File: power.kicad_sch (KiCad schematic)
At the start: 67 parts, among them J1 USB_C_Receptacle_USB2.0_14P, Q2 Q_NMOS_GDS, SW2 SW_SPDT, U12 AT24CS08-STUM, U2 BQ25895RTW, U4 LM1117DT-3.3, U5 MCP4017-xxxxLT, U6 TPS25751DREFR_C30169739, U7 LM3478MA

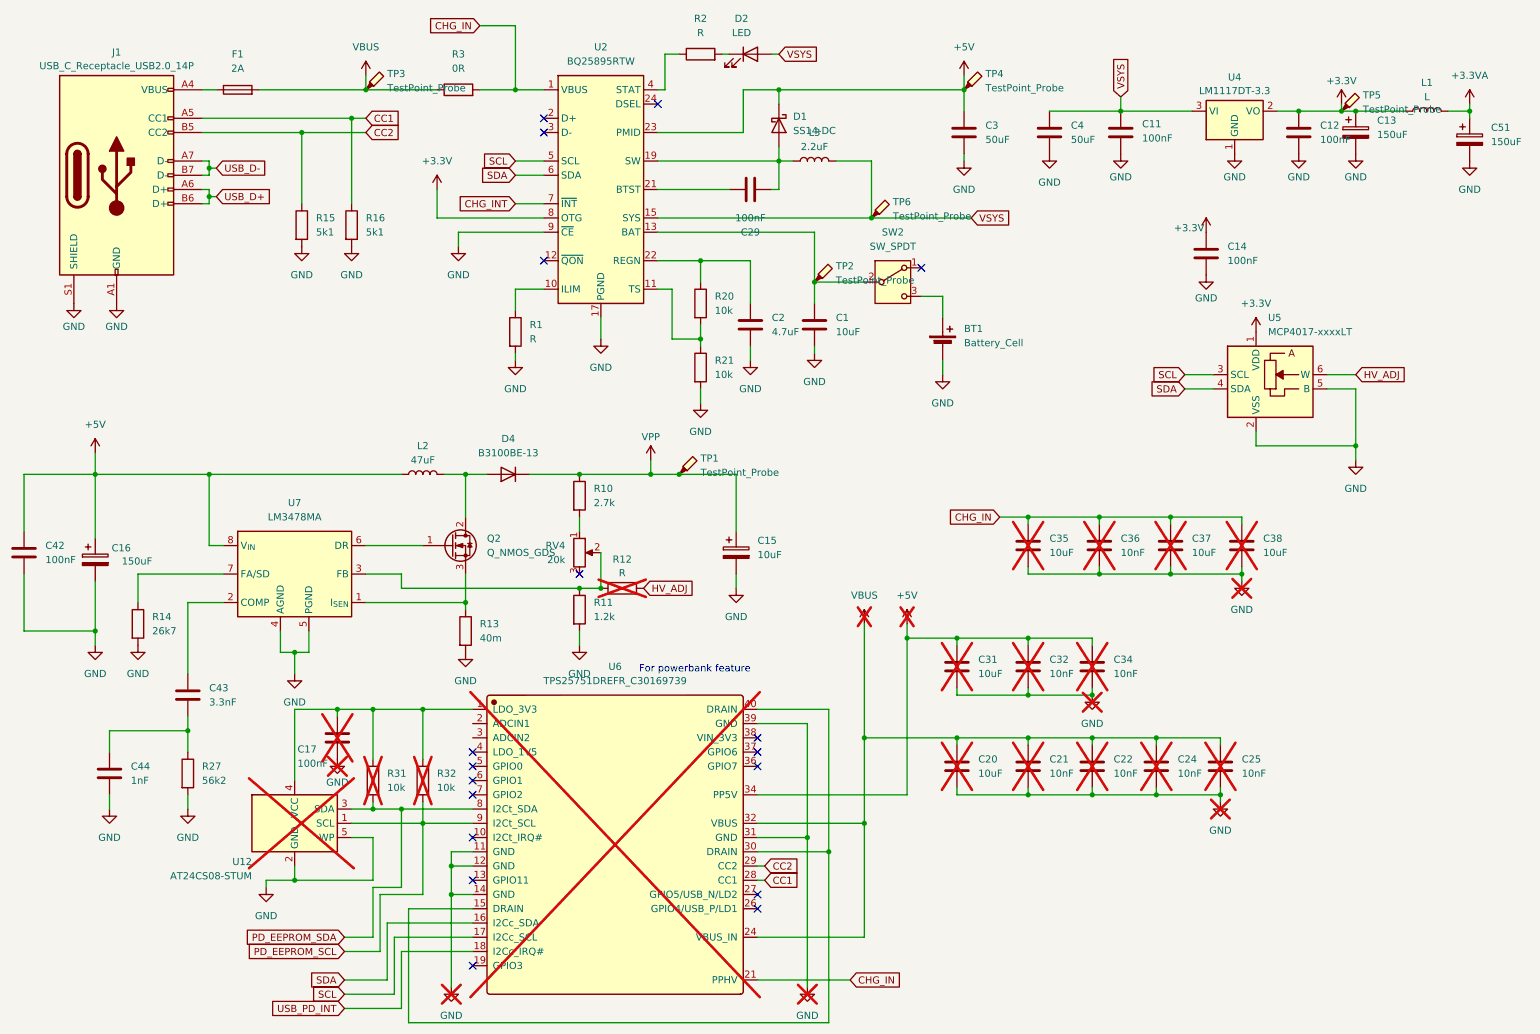
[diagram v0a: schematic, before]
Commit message: Component changes, some new feature
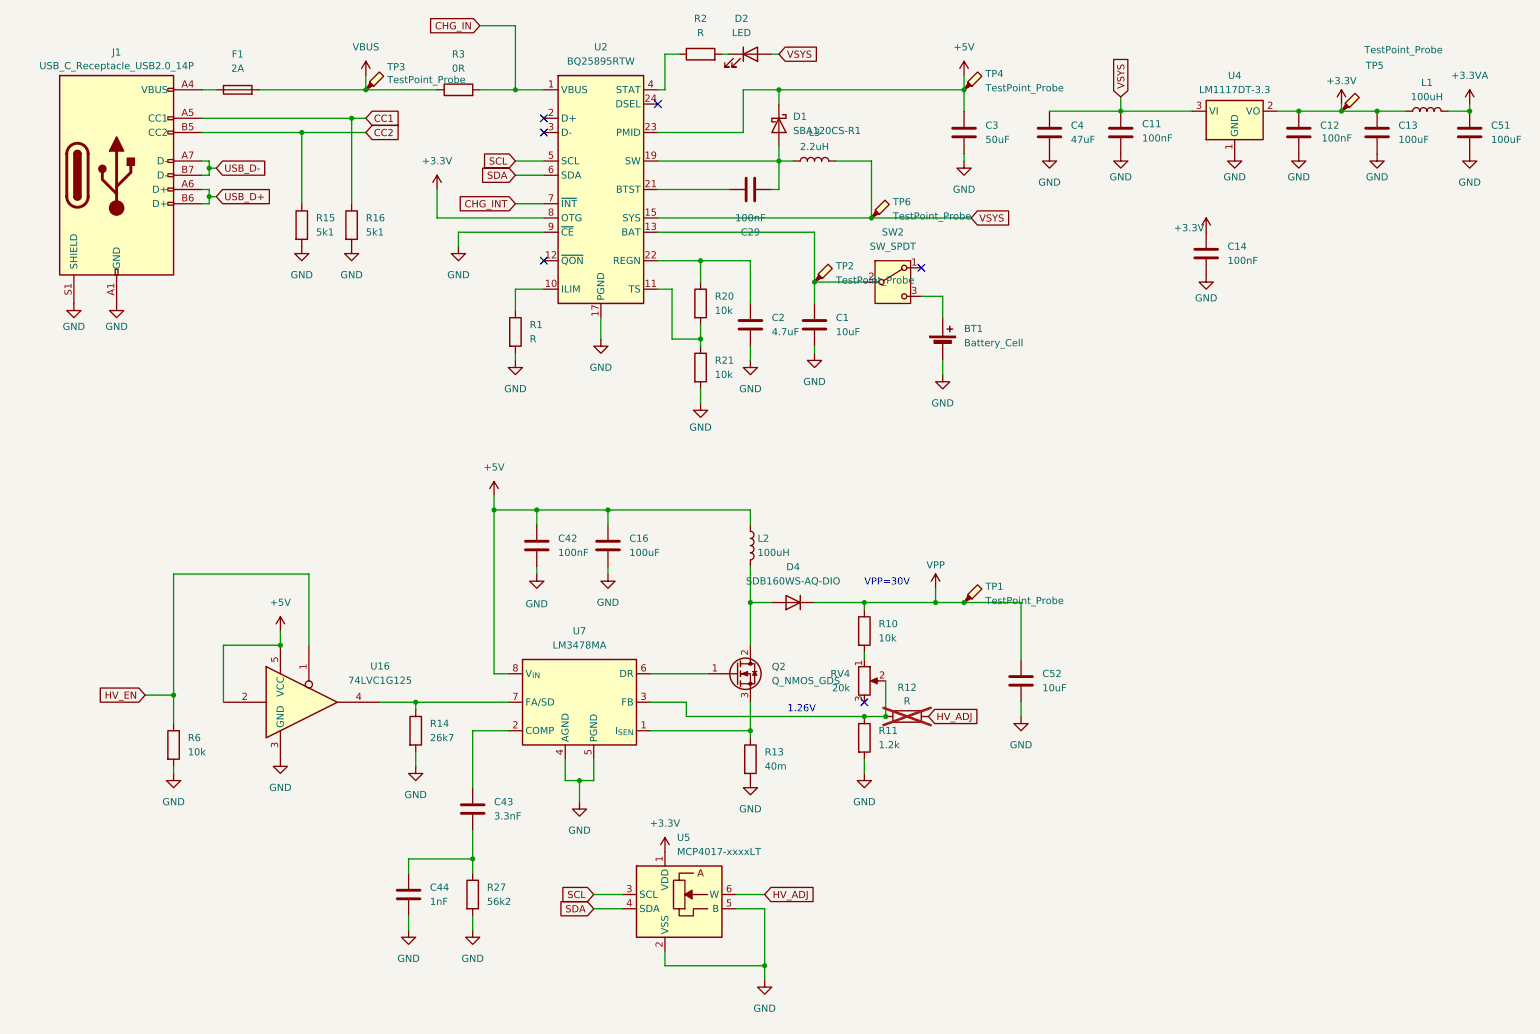
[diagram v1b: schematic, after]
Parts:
- removed C15: 10uF, Capacitor_SMD:CP_Elec_5x4.5, symbol Device:C_Polarized
- removed C16: 150uF, Capacitor_SMD:CP_Elec_5x4.5, symbol Device:C_Polarized
- removed C17: 100nF, Capacitor_SMD:C_0805_2012Metric, symbol Device:C
- removed C20, C31, C35, C37, C38: 10uF, Capacitor_SMD:C_0805_2012Metric, symbol Device:C
- removed C21, C22, C24, C25, C32, C34, C36: 10nF, Capacitor_SMD:C_0805_2012Metric, symbol Device:C
- removed R31, R32: 10k, Resistor_SMD:R_0805_2012Metric, symbol Device:R
- removed U12: AT24CS08-STUM, Package_TO_SOT_SMD:SOT-23-5, symbol Memory_EEPROM:AT24CS08-STUM
- removed U6: TPS25751DREFR_C30169739, JLCImport:TPS25751DREFR_C30169739, symbol JLCImport:TPS25751DREFR_C30169739
- added C16: 100uF, Capacitor_SMD:C_1206_3216Metric, symbol Device:C
- added C52: 10uF, Capacitor_SMD:C_1206_3216Metric, symbol Device:C
- added R6: 10k, Resistor_SMD:R_0805_2012Metric, symbol Device:R
- added U16: 74LVC1G125, Package_TO_SOT_SMD:Texas_R-PDSO-G5_DCK-5, symbol 74xGxx:74LVC1G125
- C13, C51: value 150uF -> 100uF; footprint Capacitor_SMD:CP_Elec_5x4.5 -> Capacitor_SMD:C_1206_3216Metric; symbol Device:C_Polarized -> Device:C; TME_SYMBOL EEEFT1A151AR -> CS3216X5R107M100NR
- C4: value 50uF -> 47uF; TME_SYMBOL (none) -> AMK212BC6476MG-T
- D1: value SS14-DC -> SBA120CS-R1; footprint Diode_SMD:D_SMA -> Diode_SMD:D_SOD-323; TME_SYMBOL (none) -> SBA120CS-R1
- D4: value B3100BE-13 -> SDB160WS-AQ-DIO; footprint Diode_SMD:D_SMB -> Diode_SMD:D_SOD-323; TME_SYMBOL B3100BE-13 -> SDB160WS-AQ-DIO
- L1: value L -> 100uH; footprint Inductor_SMD:L_1812_4532Metric -> Inductor_SMD:L_0805_2012Metric
- L2: value 47uF -> 100uH; Comment already have -> (none)
- L3: value 2.2uF -> 2.2uH; footprint Inductor_SMD:L_Bourns_SRP1038C_10.0x10.0mm -> Inductor_SMD:L_Taiyo-Yuden_NR-50xx; Comment already have -> (none); TME_SYMBOL PSDB1004NT101 -> DJNR5040-2R2-S; now in the parts list
- Q2: footprint Package_TO_SOT_SMD:TO-263-2 -> Package_TO_SOT_SMD:TO-252-3_TabPin2
- R10: value 2.7k -> 10k
- U4: footprint Package_TO_SOT_SMD:TO-252-3_TabPin2 -> Package_TO_SOT_SMD:SOT-223-3_TabPin2; symbol Regulator_Linear:LM1117DT-3.3 -> Regulator_Linear:LM1117MP-3.3
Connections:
- net +5V: now also C16.1, U16.2, U16.5 (VCC)
- net GND: now also C16.2, C52.2, R6.2, U16.3 (GND)
- net VPP: now also C52.1
- net at R14.1, U7.7 (FA/SD): now also U16.4
- new net HV_EN: R6.1, U16.1
- no-connect marks 18 -> 6
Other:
- note added: "1.26V"
- note added: "VPP=30V"
- note removed: "For powerbank feature"
- moved on the sheet: C42, C43, C44, D4, L2, Q2, R10, R11, R12, R13, R14, R27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
